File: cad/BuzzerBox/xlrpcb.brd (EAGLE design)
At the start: 116.2 x 162.5 mm, 12 parts, among them X1 NC3, X10 NC3, X11 B26B-PHDSS, X2 NC3, X3 NC3, X4 NC3, X5 NC3, X6 NC3, X7 NC3, X8 NC3, X9 NC3

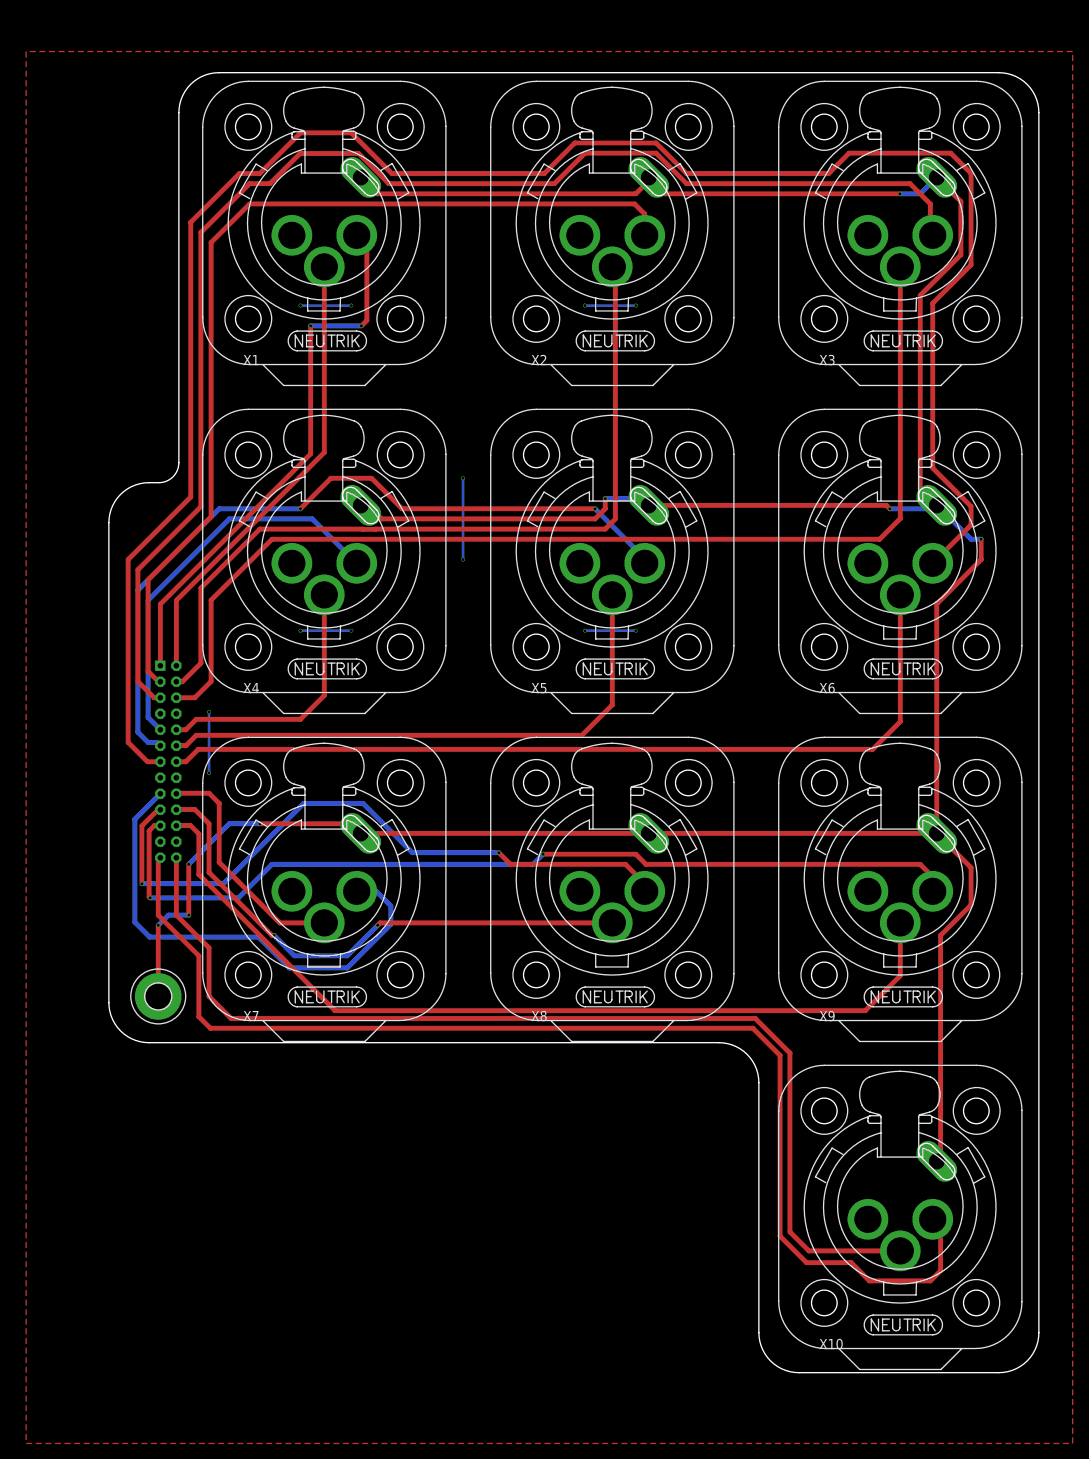
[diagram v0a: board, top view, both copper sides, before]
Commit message: V3 XLRBoard
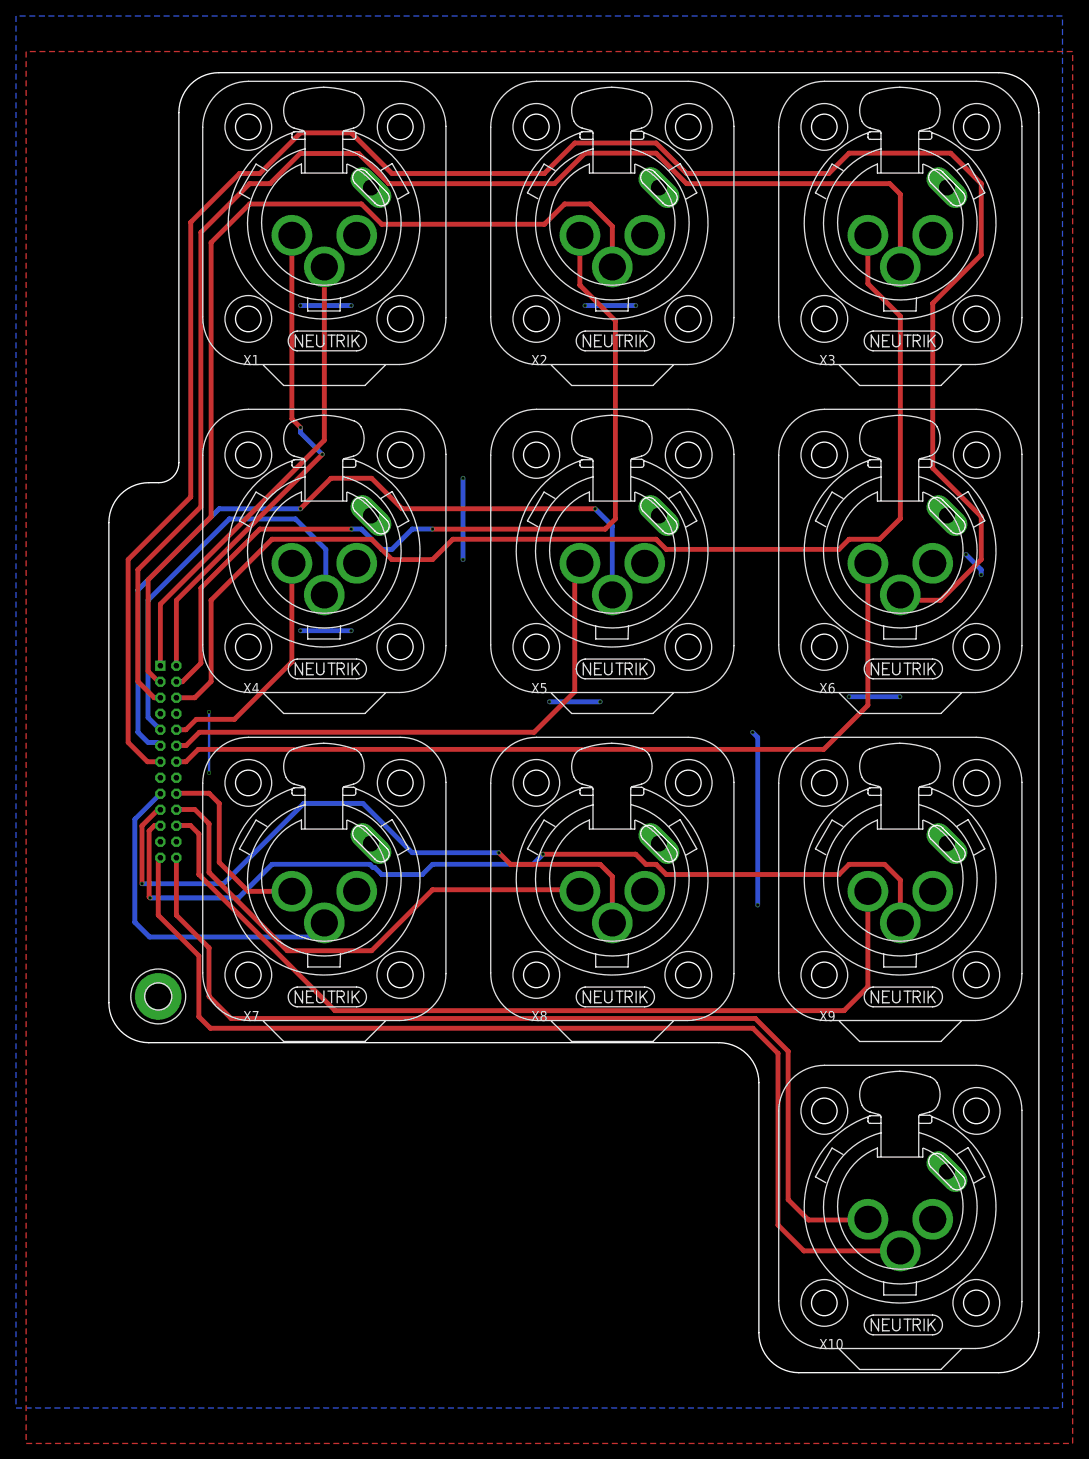
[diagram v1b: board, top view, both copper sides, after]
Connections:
- net BUZZ0: now also X10.P$1; no longer X10.P$2
- net BUZZ1: now also X1.P$1; no longer X1.P$2
- net BUZZ2: now also X2.P$1; no longer X2.P$2
- net BUZZ3: now also X3.P$1; no longer X3.P$2
- net BUZZ4: now also X4.P$1; no longer X4.P$2
- net BUZZ5: now also X5.P$1; no longer X5.P$2
- net BUZZ6: now also X6.P$1; no longer X6.P$2
- net BUZZ7: now also X7.P$1; no longer X7.P$2
- net BUZZ8: now also X8.P$1; no longer X8.P$2
- net BUZZ9: now also X9.P$1; no longer X9.P$2
- net GND: now also X1.P$3, X10.P$3, X2.P$3, X3.P$3, X4.P$3, X5.P$3, X6.P$3, X7.P$3, X8.P$3, X9.P$3; no longer X1.P$1, X10.P$1, X2.P$1, X3.P$1, X4.P$1, X5.P$1, X6.P$1, X7.P$1, X8.P$1, X9.P$1
- net LED0: now also X10.P$2; no longer X10.P$3
- net LED1: now also X1.P$2; no longer X1.P$3
- net LED2: now also X2.P$2; no longer X2.P$3
- net LED3: now also X3.P$2; no longer X3.P$3
- net LED4: now also X4.P$2; no longer X4.P$3
- net LED5: now also X5.P$2; no longer X5.P$3
- net LED6: now also X6.P$2; no longer X6.P$3
- net LED7: now also X7.P$2; no longer X7.P$3
- net LED8: now also X8.P$2; no longer X8.P$3
- net LED9: now also X9.P$2; no longer X9.P$3
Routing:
- net PE: track 402.7 -> 0.00 mm, vias 8 -> 0
- net GND: track 43.2 -> 74.7 mm, vias 12 -> 18
- net LED7: track 61.3 -> 42.6 mm
- net LED0: track 149.1 -> 134.5 mm
- net LED6: track 237.5 -> 249.1 mm
- net LED1: track 68.7 -> 58.3 mm, vias 2 -> 0
- net BUZZ3: track 137.2 -> 146.0 mm
- net BUZZ0: track 131.7 -> 123.9 mm
- net BUZZ2: track 100.5 -> 108.2 mm, vias 0 -> 2
- net BUZZ7: track 29.5 -> 23.9 mm
- net BUZZ1: track 57.5 -> 62.9 mm, vias 0 -> 2
- net BUZZ8: track 67.4 -> 64.6 mm, vias 2 -> 0
- net BUZZ4: track 32.8 -> 30.3 mm
- net LED5: track 95.3 -> 97.5 mm
- net LED9: track 113.2 -> 115.0 mm
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- added copper zone on layer 16, net PE
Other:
- board text added: "XLR-TOP-Board v3"
- board text removed: "XLR-TOP-Board v2"
